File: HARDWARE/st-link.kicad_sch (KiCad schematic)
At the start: 66 parts, among them J10 Conn_01x04_Pin, J6 USB_B_Micro, J7 Conn_01x02_Pin, J8 Conn_01x02_Pin, J9 Conn_01x06_Pin, Q1 BC848, U10 USBLC6-2SC6, U11 STM32F103CBTx, U12 LD3985M33R_SOT23, Y4 8 MHz

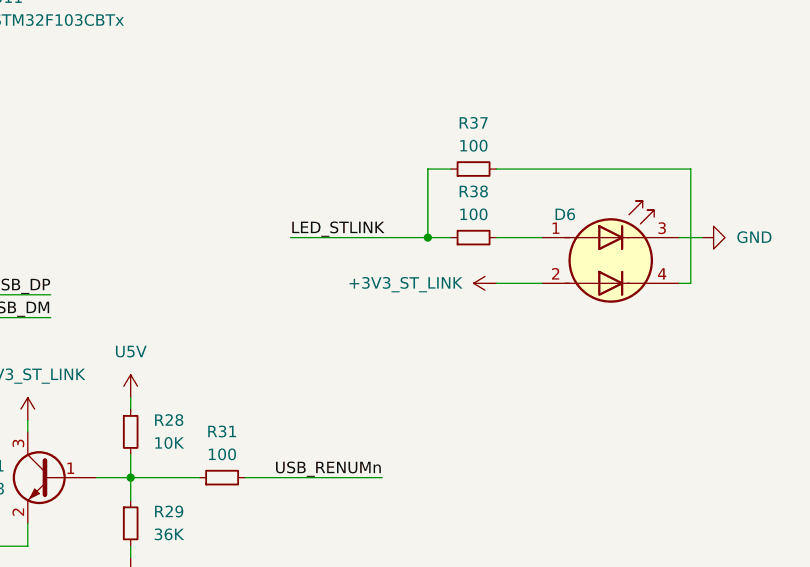
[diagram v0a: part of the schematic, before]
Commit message: tracerouting
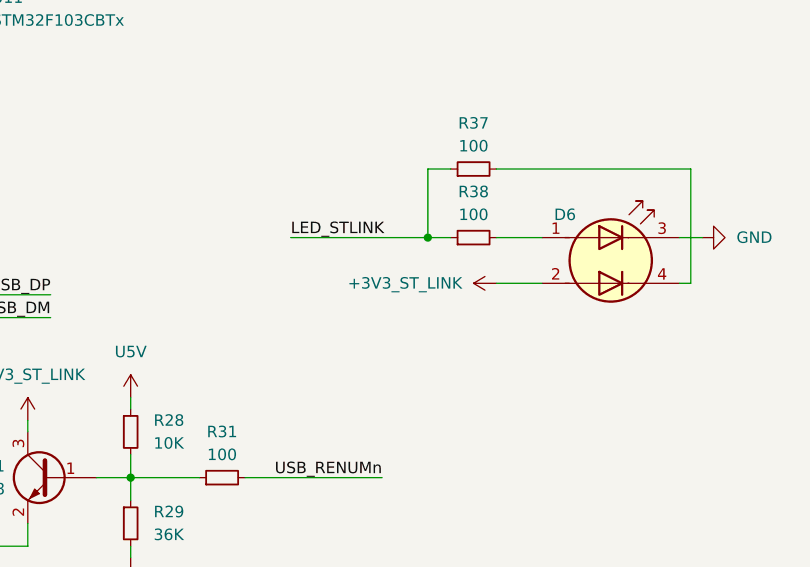
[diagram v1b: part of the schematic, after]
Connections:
- net +3V3 renamed +3V3_ST_LINK
- net +3V3_ST_LINK: no longer R23.2
- net +5V0 renamed U5V
- net U5V: no longer D8.2 (A), D9.2 (A)
- new net +3V3_PER: R23.2
- new net E5V: D9.2 (A)
- new net VIN_5V: D8.2 (A)
